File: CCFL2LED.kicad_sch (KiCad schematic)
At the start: 68 parts, among them J2 USB_C_Receptacle_USB2.0_16P, J3 Jack-DC, J4 OUTPUT, J5 Conn_01x02_Pin, J6 Conn_01x02_Pin, J7 Conn_01x02_Pin, Q1 S8050, SW1 SW_SPDT, U1 PT4115, U2 PT4115, U3 AP62201WU-7, U7 LM2596 Modul, U8 AMS1117-3.3, U9 CH224K

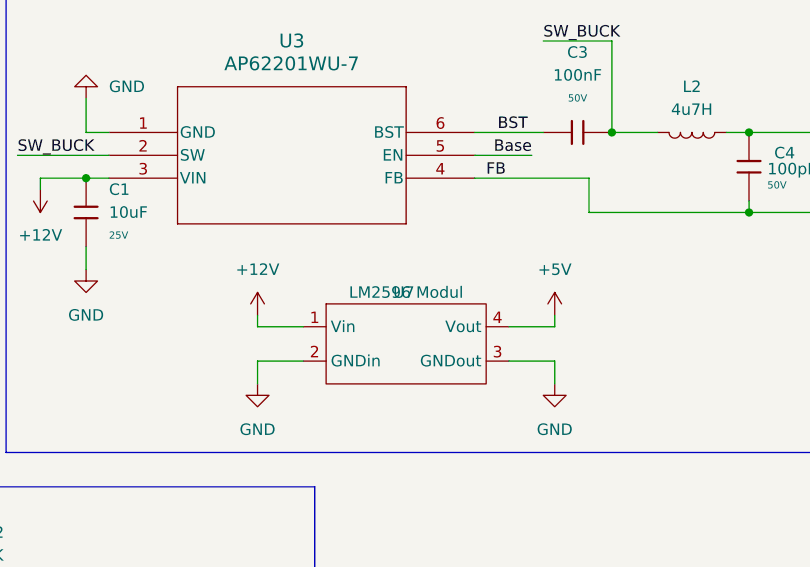
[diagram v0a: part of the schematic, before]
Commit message: Update schematic and pictures
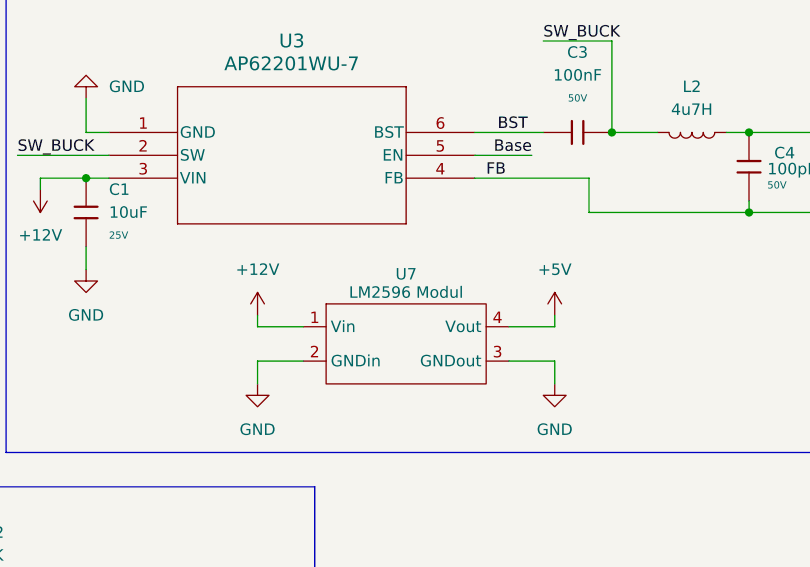
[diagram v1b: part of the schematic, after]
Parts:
- J3: LCSC Part # C3010534 -> C720557
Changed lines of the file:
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@@
 			)
 		)
-		(property "LCSC Part #" "C3010534"
+		(property "LCSC Part #" "C720557"
 			(at 149.86 27.94 0)
 			(effects
@@
 		(dnp no)
 		(property "Reference" "U7"
-			(at 181.356 146.05 0)
+			(at 181.61 144.018 0)
 			(effects
 				(font
